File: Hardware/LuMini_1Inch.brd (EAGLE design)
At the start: 28.7 x 43.2 mm, 48 parts, among them J1 DOUBLE_LED_PAD, J2 DOUBLE_LED_PAD, J4 DOUBLE_LED_PAD

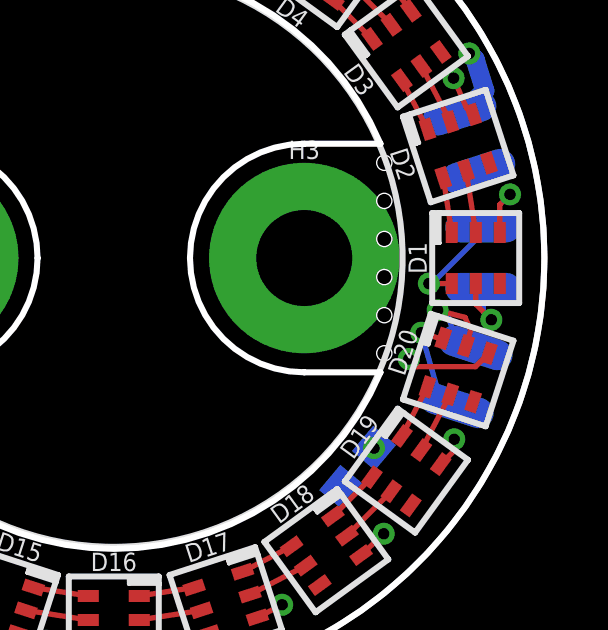
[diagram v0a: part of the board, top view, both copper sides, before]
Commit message: qc checklist changes
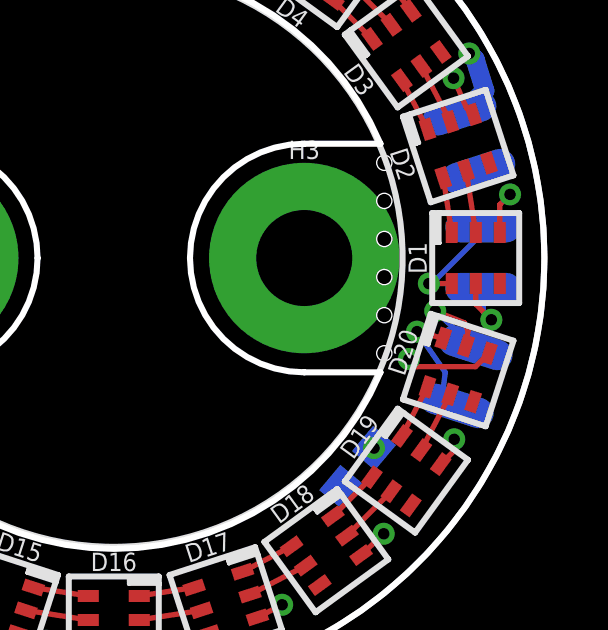
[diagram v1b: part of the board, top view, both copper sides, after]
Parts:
- D1, D10, D11, D12, D13, D14, D15, D16, D17, D18, D19, D2, D20, D3, D4, D5, D6, D7, D8, D9: value APA1022020 -> APA102-2020
- H1, H2, H3, H4: value STANDOFF_ELECTRICALSTANDOFF-ELECTRICAL-NOTHERMALS -> STANDOFF_ELECTRICAL-NOTHERMALS
- J1, J2, J4: value DOUBLE_LED_PAD -> SOLDER_PAD_2; device Andy:DOUBLELEDPAD -> SparkFun-Connectors:SOLDER_PAD_2
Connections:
- net N$2 renamed CI
- net N$3 renamed DI
- net N$41 renamed CO
- net N$42 renamed DO
